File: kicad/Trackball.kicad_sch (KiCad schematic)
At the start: 40 parts, among them J1 Conn_01x04, J2 Conn_02x10_Odd_Even, SW1 SW_Push, SW2 SW_Push, U1 TCR2EF19, U2 PMW3360, U3 RP2040, U4 TLV73333PDBV, U5 W25Q128JVS, Y1 Crystal_GND24

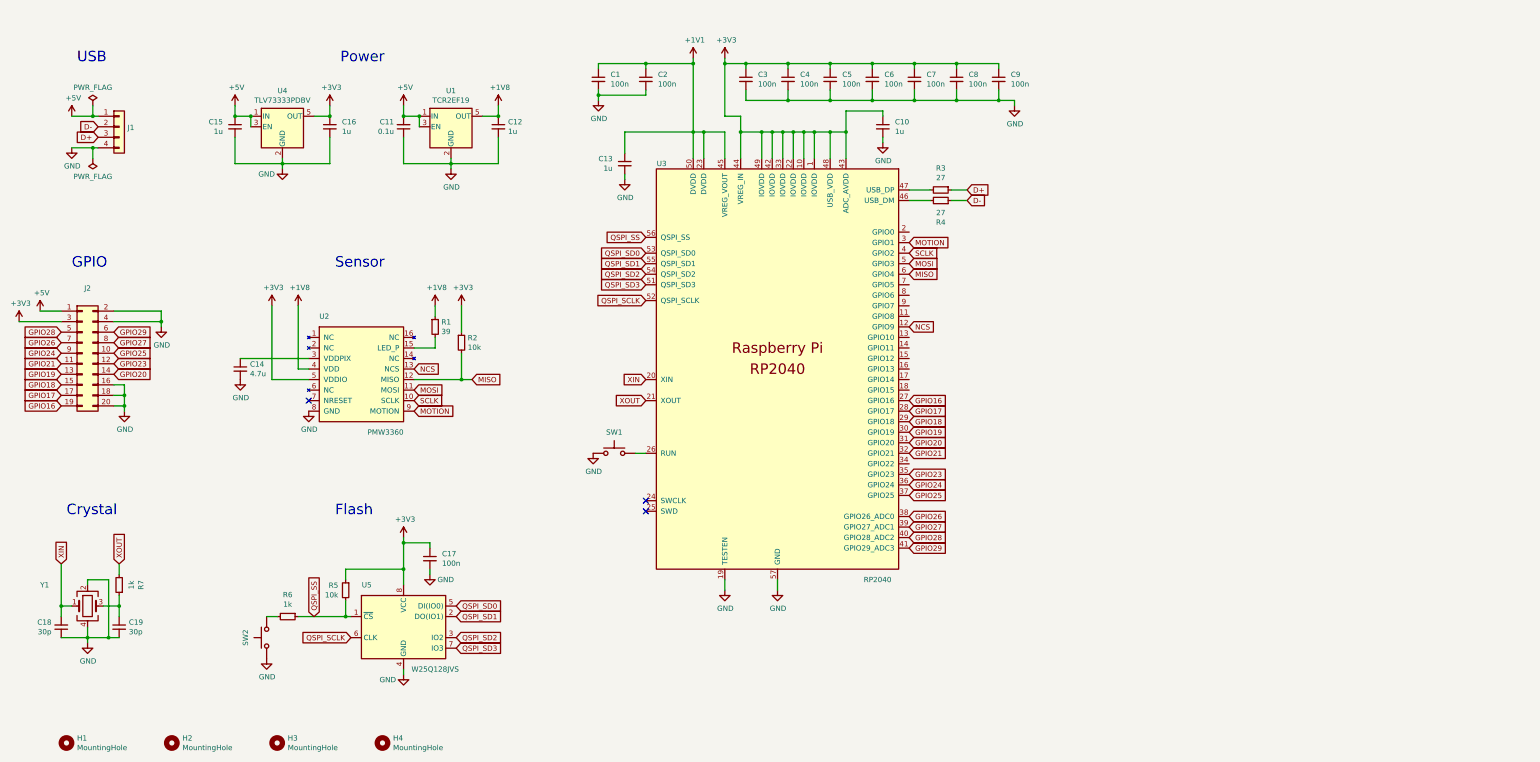
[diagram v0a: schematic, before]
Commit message: up
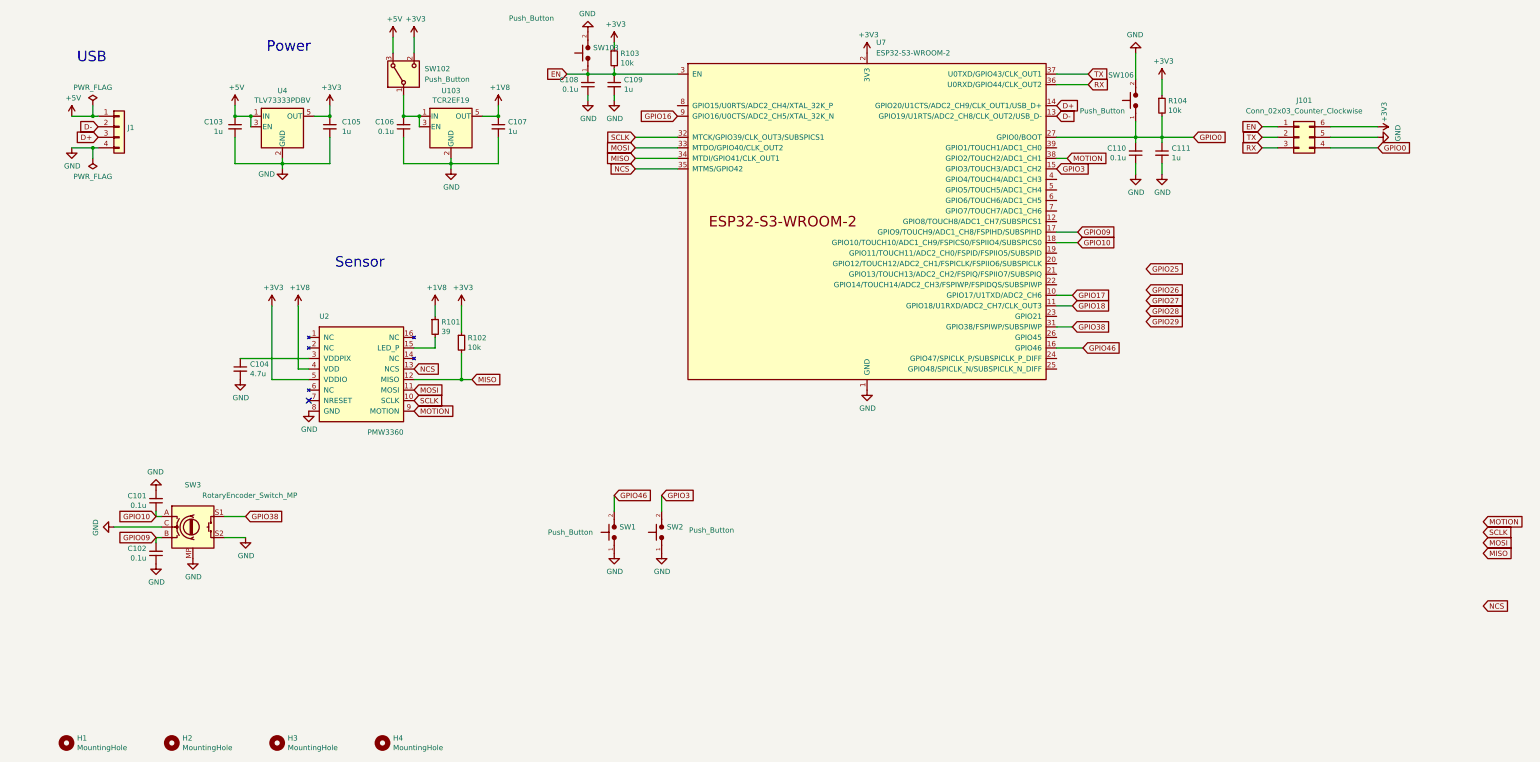
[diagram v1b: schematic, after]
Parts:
- removed C1, C17, C2, C3, C4, C5, C6, C7, C8, C9: 100n, Capacitor_SMD:C_0402_1005Metric, symbol Device:C_Small
- removed C10, C13: 1u, Capacitor_SMD:C_0402_1005Metric, symbol Device:C_Small
- removed C18, C19: 30p, Capacitor_SMD:C_0402_1005Metric, symbol Device:C_Small
- removed J2: Conn_02x10_Odd_Even, Connector_PinHeader_2.54mm:PinHeader_2x10_P2.54mm_Vertical, symbol Connector_Generic:Conn_02x10_Odd_Even
- removed R3, R4: 27, Resistor_SMD:R_0402_1005Metric, symbol Device:R_Small
- removed R5: 10k, Resistor_SMD:R_0402_1005Metric, symbol Device:R_Small
- removed R6, R7: 1k, Resistor_SMD:R_0402_1005Metric, symbol Device:R_Small
- removed SW1, SW2: SW_Push, Button_Switch_SMD:SW_SPST_Omron_B3FS-100xP, symbol Switch:SW_Push
- removed U3: RP2040, RP2040:RP2040-QFN-56, symbol RP2040:RP2040
- removed U5: W25Q128JVS, Package_SO:SOIC-8_5.23x5.23mm_P1.27mm, symbol Trackball-rescue:W25Q128JVS-Memory_Flash
- removed Y1: Crystal_GND24, Crystal:Crystal_SMD_3225-4Pin_3.2x2.5mm, symbol Device:Crystal_GND24
- added C101, C102, C108, C110: 0.1u, Capacitor_SMD:C_0805_2012Metric, symbol Device:C_Small
- added C109, C111: 1u, Capacitor_SMD:C_0805_2012Metric, symbol Device:C_Small
- added J101: Conn_02x03_Counter_Clockwise, Connector_Harwin:Harwin_Gecko-G125-FVX0605L0X_2x03_P1.25mm_Vertical, symbol Connector_Generic:Conn_02x03_Counter_Clockwise
- added R103, R104: 10k, Resistor_SMD:R_0805_2012Metric, symbol Device:R_Small
- added SW1, SW2: Push_Button, PCM_Switch_Keyboard_Hotswap_Kailh:SW_Hotswap_Kailh_Choc_V1V2_1.00u, symbol PCM_SL_Devices:Push_Button
- added SW102: Push_Button, PCM_4ms_Switch:Switch_Toggle_SPDT_SubMini, symbol Switch:SW_Wuerth_450301014042
- added SW103, SW106: Push_Button, Button_Switch_SMD:SW_Push_1P1T_NO_CK_KSC7xxJ, symbol PCM_SL_Devices:Push_Button
- added SW3: RotaryEncoder_Switch_MP, PMW3360:RollerEncoder_Panasonic_EVQWGD001, symbol Device:RotaryEncoder_Switch_MP
- added U7: ESP32-S3-WROOM-2, PCM_Espressif:ESP32-S3-WROOM-2, symbol PCM_Espressif:ESP32-S3-WROOM-2
- C103: renamed from C15; footprint Capacitor_SMD:C_0402_1005Metric -> Capacitor_SMD:C_0805_2012Metric
- C104: renamed from C14; footprint Capacitor_SMD:C_0402_1005Metric -> Capacitor_SMD:C_0805_2012Metric
- C105: renamed from C16; footprint Capacitor_SMD:C_0402_1005Metric -> Capacitor_SMD:C_0805_2012Metric
- C106: renamed from C11; footprint Capacitor_SMD:C_0603_1608Metric -> Capacitor_SMD:C_0805_2012Metric
- C107: renamed from C12; footprint Capacitor_SMD:C_0603_1608Metric -> Capacitor_SMD:C_0805_2012Metric
- R101: renamed from R1; footprint Resistor_SMD:R_0402_1005Metric -> Resistor_SMD:R_0805_2012Metric
- R102: renamed from R2; footprint Resistor_SMD:R_0402_1005Metric -> Resistor_SMD:R_0805_2012Metric
- renumbered U1 to U103
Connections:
- net +3V3: now also J101.6 (Pin_6), R103.1, R104.1, SW102.2 (C), U7.2 (3V3)
- net +5V: now also SW102.3 (A); no longer C106.2, U103.1 (IN), U103.3 (EN)
- net D+: now also U7.14 (GPIO20/U1CTS/ADC2_CH9/CLK_OUT1/USB_D+)
- net D-: now also U7.13 (GPIO19/U1RTS/ADC2_CH8/CLK_OUT2/USB_D-)
- net GND: now also C101.2, C102.1, C108.1, C109.2, C110.1, C111.2, J101.5 (Pin_5), SW1.1, SW103.2, SW106.2, SW2.1, SW3.C, SW3.MP, SW3.S2, U7.1 (GND), U7.40 (GND), U7.41 (GND)
- net GPIO16: now also U7.9 (GPIO16/U0CTS/ADC2_CH5/XTAL_32K_N)
- net GPIO17: now also U7.10 (GPIO17/U1TXD/ADC2_CH6)
- net GPIO18: now also U7.11 (GPIO18/U1RXD/ADC2_CH7/CLK_OUT3)
- net MISO: now also U7.34 (MTDI/GPIO41/CLK_OUT1)
- net MOSI: now also U7.33 (MTDO/GPIO40/CLK_OUT2)
- net MOTION: now also U7.38 (GPIO2/TOUCH2/ADC1_CH1)
- net NCS: now also U7.35 (MTMS/GPIO42)
- net SCLK: now also U7.32 (MTCK/GPIO39/CLK_OUT3/SUBSPICS1)
- new net: C106.2, SW102.1 (B), U103.1 (IN), U103.3 (EN)
- new net EN: C108.2, C109.1, J101.1 (Pin_1), R103.2, SW103.1, U7.3 (EN)
- new net GPIO0: C110.2, C111.1, J101.4 (Pin_4), R104.2, SW106.1, U7.27 (GPIO0/BOOT)
- new net GPIO09: C102.2, SW3.B, U7.17 (GPIO9/TOUCH9/ADC1_CH8/FSPIHD/SUBSPIHD)
- new net GPIO10: C101.1, SW3.A, U7.18 (GPIO10/TOUCH10/ADC1_CH9/FSPICS0/FSPIIO4/SUBSPICS0)
- new net GPIO3: SW2.2, U7.15 (GPIO3/TOUCH3/ADC1_CH2)
- new net GPIO38: SW3.S1, U7.31 (GPIO38/FSPIWP/SUBSPIWP)
- new net GPIO46: SW1.2, U7.16 (GPIO46)
- new net RX: J101.3 (Pin_3), U7.36 (U0RXD/GPIO44/CLK_OUT2)
- new net TX: J101.2 (Pin_2), U7.37 (U0TXD/GPIO43/CLK_OUT1)
- no-connect marks 3 -> 1
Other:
- note removed: "Crystal"
- note removed: "Flash"
- note removed: "GPIO"
